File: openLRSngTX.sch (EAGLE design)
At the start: 28 parts, among them IC1 RFM23BPSMD, J1 AVR_SPI_PRG_6PTH, Q1 MMBT2222, U1 ATMEGA328P, X1 BU-SMA-V, Y1 16MHz

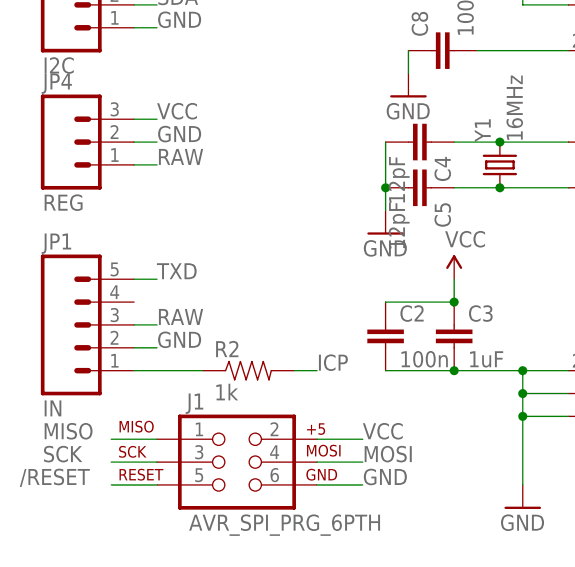
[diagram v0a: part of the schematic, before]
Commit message: minor updates
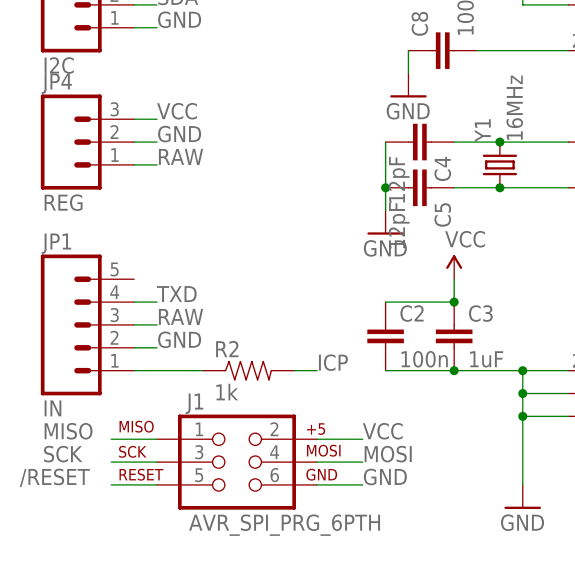
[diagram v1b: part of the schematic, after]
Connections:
- net TXD: now also JP1.4; no longer JP1.5
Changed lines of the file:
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@@
 </segment>
 <segment>
-<pinref part="JP1" gate="G$1" pin="5"/>
-<wire x1="-5.08" y1="50.8" x2="-2.54" y2="50.8" width="0.1524" layer="91"/>
-<label x="-2.54" y="50.8" size="1.778" layer="95"/>
+<pinref part="JP1" gate="G$1" pin="4"/>
+<wire x1="-5.08" y1="48.26" x2="-2.54" y2="48.26" width="0.1524" layer="91"/>
+<label x="-2.54" y="48.26" size="1.778" layer="95"/>
 </segment>
 </net>
